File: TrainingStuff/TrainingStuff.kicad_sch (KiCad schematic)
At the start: 0 parts

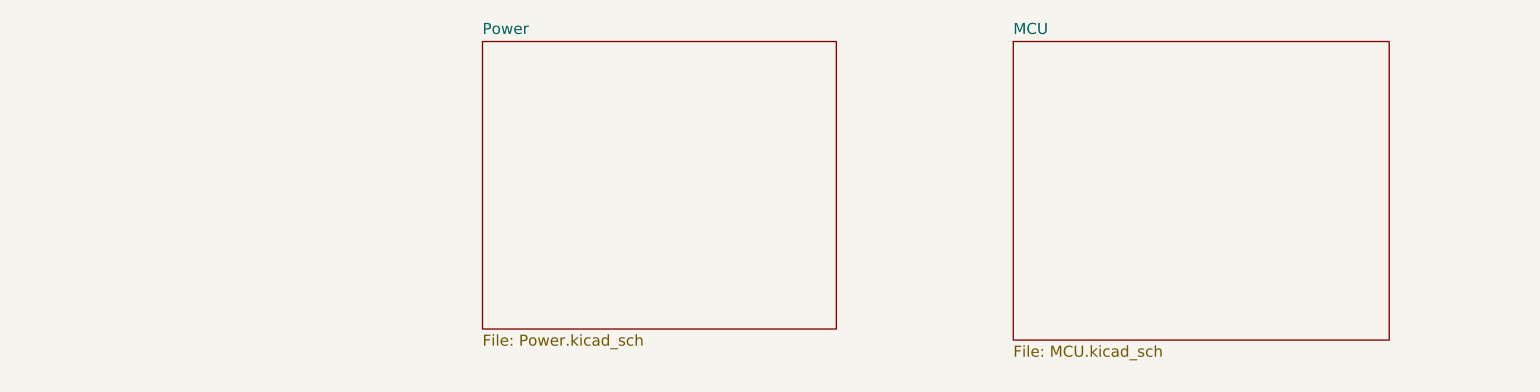
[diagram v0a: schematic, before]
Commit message: Add Schematic
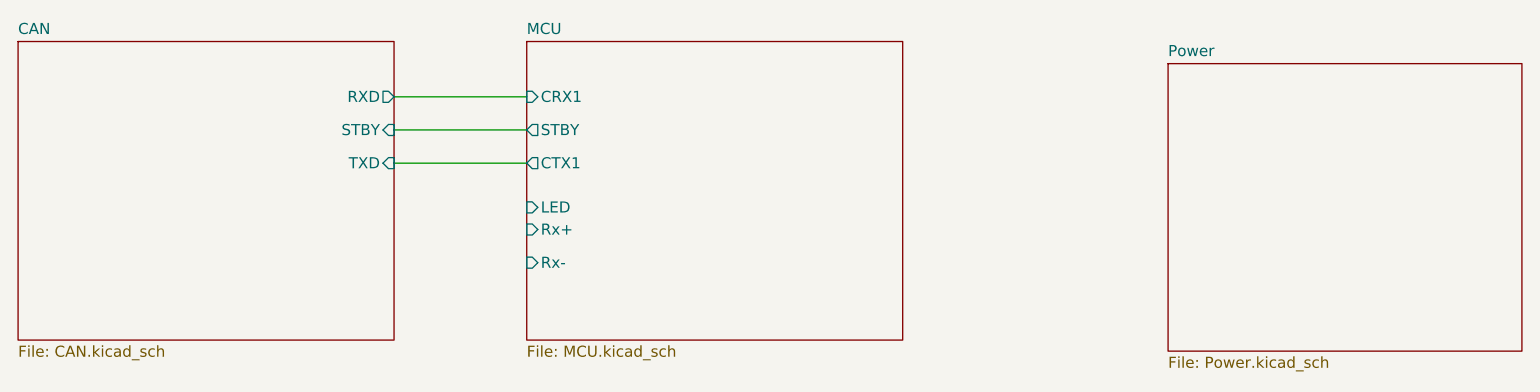
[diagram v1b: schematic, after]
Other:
- added sheet CAN (CAN.kicad_sch)
- sheet MCU ports: added CRX1, CTX1, LED, Rx+, Rx-, STBY; removed none
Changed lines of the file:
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@@
 	(generator_version "9.0")
 	(paper "A4")
+	(wire
+		(pts
+			(xy 74.93 88.9) (xy 90.17 88.9)
+		)
+		(stroke
+			(width 0)
+			(type default)
+		)
+	)
+	(wire
+		(pts
+			(xy 74.93 85.09) (xy 90.17 85.09)
+		)
+		(stroke
+			(width 0)
+			(type default)
+		)
+	)
+	(wire
+		(pts
+			(xy 74.93 81.28) (xy 90.17 81.28)
+		)
+		(stroke
+			(width 0)
+			(type default)
+		)
+	)
 	(sheet
-		(at 85.09 74.93)
+		(at 163.83 77.47)
 		(size 40.64 33.02)
 		(exclude_from_sim no)
@@
 		)
 		(property "Sheetname" "Power"
-			(at 85.09 74.2184 0)
+			(at 163.83 76.7584 0)
 			(effects
 				(font
@@
 		)
 		(property "Sheetfile" "Power.kicad_sch"
-			(at 85.09 108.5346 0)
+			(at 163.83 111.0746 0)
 			(effects
 				(font
@@
 	)
 	(sheet
-		(at 146.05 74.93)
+		(at 31.75 74.93)
 		(size 43.18 34.29)
 		(exclude_from_sim no)
@@
 			(color 0 0 0 0.0000)
 		)
+		(property "Sheetname" "CAN"
+			(at 31.75 74.2184 0)
+			(effects
+				(font
+					(size 1.27 1.27)
+				)
+				(justify left bottom)
+			)
+		)
+		(property "Sheetfile" "CAN.kicad_sch"
+			(at 31.75 109.8046 0)
+			(effects
+				(font
+					(size 1.27 1.27)
+				)
+				(justify left top)
+			)
+		)
+		(pin "RXD" output
+			(at 74.93 81.28 0)
+			(effects
+				(font
+					(size 1.27 1.27)
+				)
+				(justify right)
+			)
+		)
+		(pin "STBY" input
+			(at 74.93 85.09 0)
+			(effects
+				(font
+					(size 1.27 1.27)
+				)
+				(justify right)
+			)
+		)
+		(pin "TXD" input
+			(at 74.93 88.9 0)
+			(effects
+				(font
+					(size 1.27 1.27)
+				)
+				(justify right)
+			)
+		)
+		(instances
+			(project "TrainingStuff"
+				(path "/7bedb2c1-4b41-4164-a76e-e6479fce2d5a"
+					(page "4")
+				)
+			)
+		)
+	)
+	(sheet
+		(at 90.17 74.93)
+		(size 43.18 34.29)
+		(exclude_from_sim no)
+		(in_bom yes)
+		(on_board yes)
+		(dnp no)
+		(fields_autoplaced yes)
+		(stroke
+			(width 0.1524)
+			(type solid)
+		)
+		(fill
+			(color 0 0 0 0.0000)
+		)
 		(property "Sheetname" "MCU"
-			(at 146.05 74.2184 0)
+			(at 90.17 74.2184 0)
 			(effects
 				(font
@@
 		)
 		(property "Sheetfile" "MCU.kicad_sch"
-			(at 146.05 109.8046 0)
+			(at 90.17 109.8046 0)
 			(effects
 				(font
@@
 			)
 		)
+		(pin "CRX1" input
+			(at 90.17 81.28 180)
+			(effects
+				(font
+					(size 1.27 1.27)
+				)
+				(justify left)
+			)
+		)
+		(pin "CTX1" output
+			(at 90.17 88.9 180)
+			(effects
+				(font
+					(size 1.27 1.27)
+				)
+				(justify left)
+			)
+		)
+		(pin "LED" input
+			(at 90.17 93.98 180)
+			(effects
+				(font
+					(size 1.27 1.27)
+				)
+				(justify left)
+			)
+		)
+		(pin "Rx+" input
+			(at 90.17 96.52 180)
+			(effects
+				(font
+					(size 1.27 1.27)
+				)
+				(justify left)
+			)
+		)
+		(pin "Rx-" input
+			(at 90.17 100.33 180)
+			(effects
+				(font
+					(size 1.27 1.27)
+				)
+				(justify left)
+			)
+		)
+		(pin "STBY" output
+			(at 90.17 85.09 180)
+			(effects
+				(font
+					(size 1.27 1.27)
+				)
+				(justify left)
+			)
+		)
